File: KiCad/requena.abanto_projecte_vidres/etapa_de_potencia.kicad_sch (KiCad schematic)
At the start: 19 parts, among them J5 Conn_01x02, P1 282837-2, P2 282837-2, U1 L298N, U2 TSR2-2450, U3 MCP6022, U4 LM1117DT-3.3

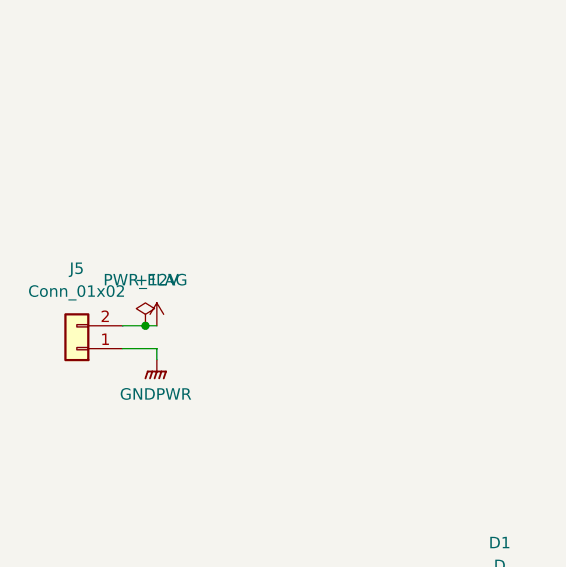
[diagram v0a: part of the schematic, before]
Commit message: primera pcb
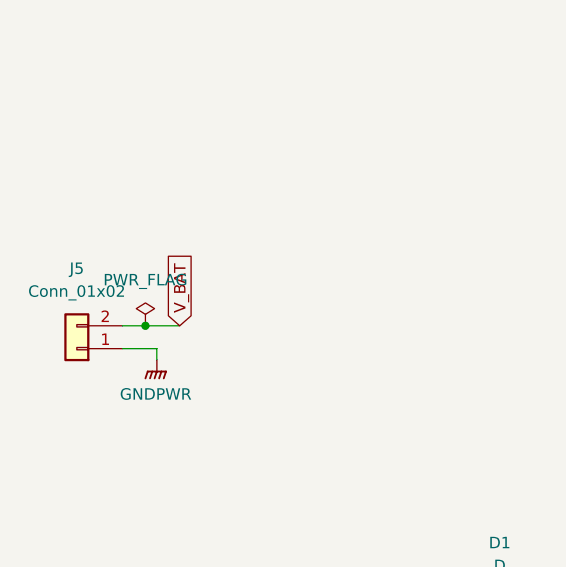
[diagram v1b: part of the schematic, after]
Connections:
- net +12V: no longer J5.2 (Pin_2)
- net V_BAT: now also J5.2 (Pin_2)
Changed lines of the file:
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@@
 	(wire
 		(pts
-			(xy 31.75 96.52) (xy 33.02 96.52)
+			(xy 31.75 96.52) (xy 35.56 96.52)
 		)
 		(stroke
@@
 		(property "Intersheetrefs" "${INTERSHEET_REFS}"
 			(at 208.28 73.3962 90)
+			(effects
+				(font
+					(size 1.27 1.27)
+				)
+				(justify left)
+				(hide yes)
+			)
+		)
+	)
+	(global_label "V_BAT"
+		(shape input)
+		(at 35.56 96.52 90)
+		(fields_autoplaced yes)
+		(effects
+			(font
+				(size 1.27 1.27)
+			)
+			(justify left)
+		)
+		(property "Intersheetrefs" "${INTERSHEET_REFS}"
+			(at 35.56 88.1524 90)
 			(effects
 				(font
@@
 					(unit 1)
 				)
-			)
-		)
-	)
-	(symbol
-		(lib_id "power:+12V")
-		(at 33.02 96.52 0)
-		(unit 1)
-		(exclude_from_sim no)
-		(in_bom yes)
-		(on_board yes)
-		(dnp no)
-		(fields_autoplaced yes)
-		(property "Reference" "#PWR02"
-			(at 33.02 100.33 0)
-			(effects
-				(font
-					(size 1.27 1.27)
-				)
-				(hide yes)
-			)
-		)
-		(property "Value" "+12V"
-			(at 33.02 91.44 0)
-			(effects
-				(font
-					(size 1.27 1.27)
-				)
-			)
-		)
-		(property "Footprint" ""
-			(at 33.02 96.52 0)
-			(effects
-				(font
-					(size 1.27 1.27)
-				)
-				(hide yes)
-			)
-		)
-		(property "Datasheet" ""
-			(at 33.02 96.52 0)
-			(effects
-				(font
-					(size 1.27 1.27)
-				)
-				(hide yes)
-			)
-		)
-		(property "Description" "Power symbol creates a global label with name \"+12V\""
-			(at 33.02 96.52 0)
-			(effects
-				(font
-					(size 1.27 1.27)
-				)
-				(hide yes)
-			)
-		)
-		(pin "1"
-		)
-		(instances
-			(project ""
-				(path "/4006572a-320d-4ed7-bf52-f860e1c069c6/0b0d2692-6fb2-4ddb-9a32-8981b2e43675"
-					(reference "#PWR02")
-					(unit 1)
-				)
